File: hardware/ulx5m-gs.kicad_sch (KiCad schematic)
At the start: 4 parts

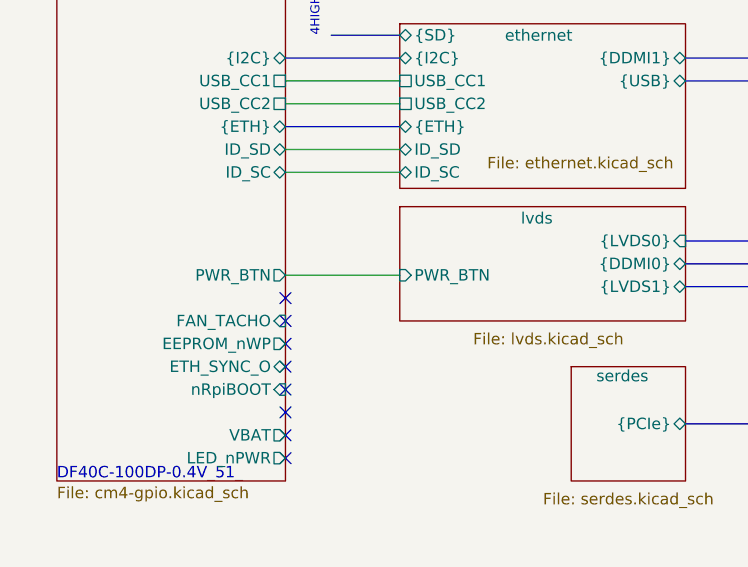
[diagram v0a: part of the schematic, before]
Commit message: CleanUP
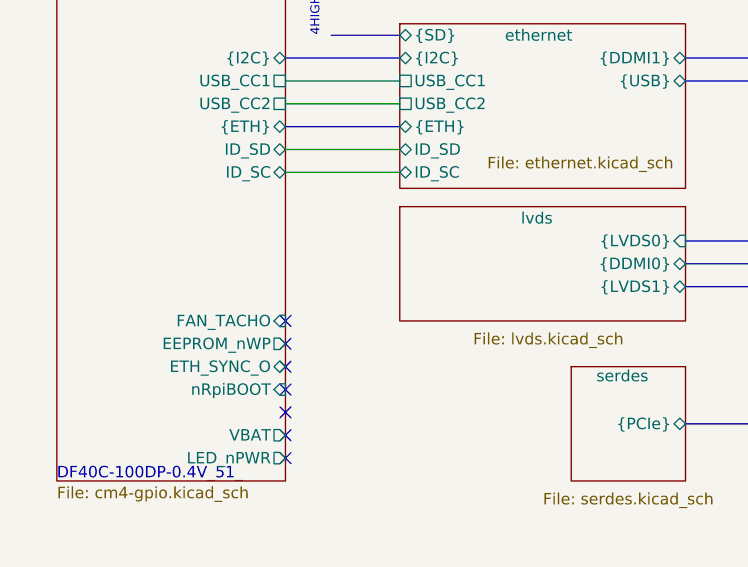
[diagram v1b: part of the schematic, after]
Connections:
- no-connect marks 8 -> 7
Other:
- sheet cm4-gpio ports: added none; removed PWR_BTN
- sheet lvds ports: added none; removed PWR_BTN
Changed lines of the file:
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@@
-	)
-	(no_connect
-		(at 45.72 107.95)
 	)
 	(no_connect
@@
 			(width 0)
 			(type default)
-		)
-	)
-	(wire
-		(pts
-			(xy 45.72 105.41) (xy 58.42 105.41)
-		)
-		(stroke
-			(width 0)
-			(type default)
-			(color 255 0 255 1)
 		)
 	)
@@
 			)
 		)
-		(pin "PWR_BTN" output
-			(at 45.72 105.41 0)
-			(effects
-				(font
-					(size 1.27 1.27)
-				)
-				(justify right)
-			)
-		)
 		(pin "USB_CC1" passive
 			(at 45.72 83.82 0)
@@
 			)
 		)
-		(pin "PWR_BTN" input
-			(at 58.42 105.41 180)
-			(effects
-				(font
-					(size 1.27 1.27)
-				)
-				(justify left)
-			)
-		)
